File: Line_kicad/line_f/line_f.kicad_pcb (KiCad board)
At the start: 2 copper layers, 137.5 x 154 mm, 15 parts, among them M2 Motor_DC, M3 Motor_DC, SW1 SW_SPST, SW2 SW_SPDT, SW3 SW_Push, SW4 SW_Push, U1 TB6612FNG_LINE, m1 BLACKPILL

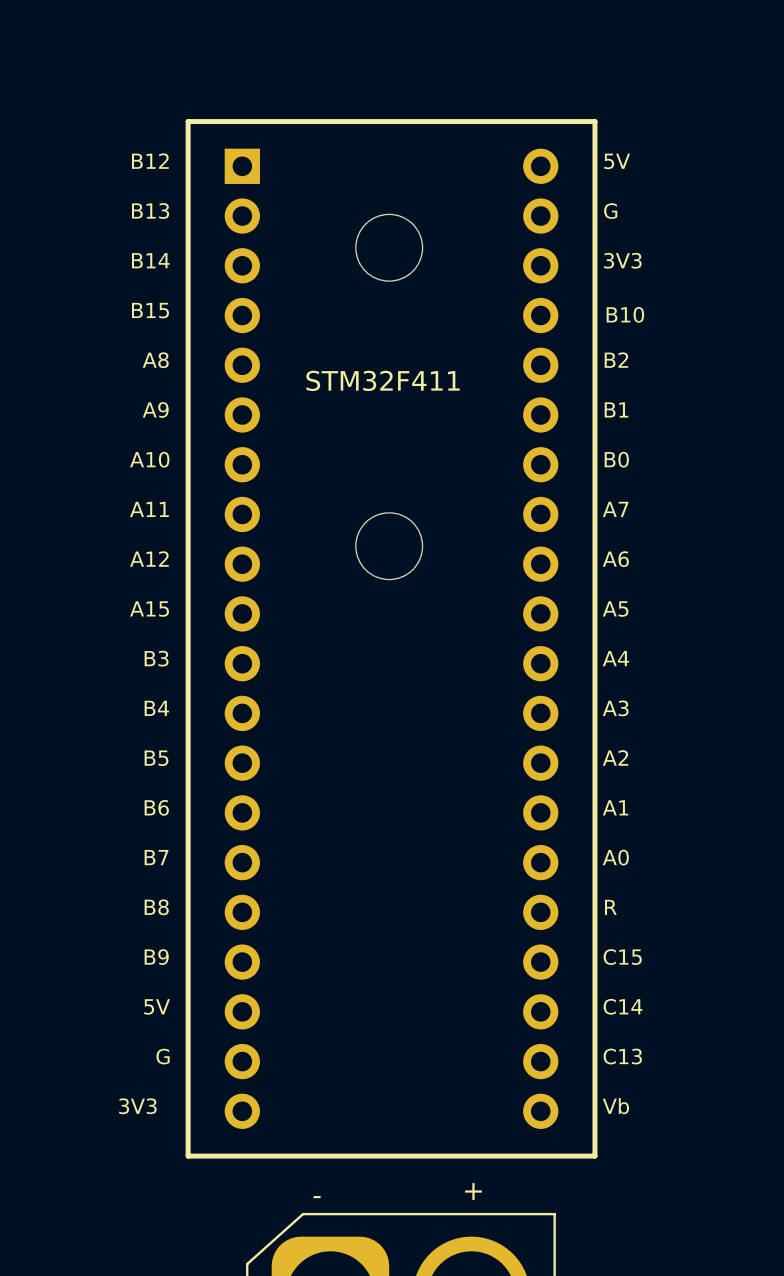
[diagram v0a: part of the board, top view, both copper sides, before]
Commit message: v9.0
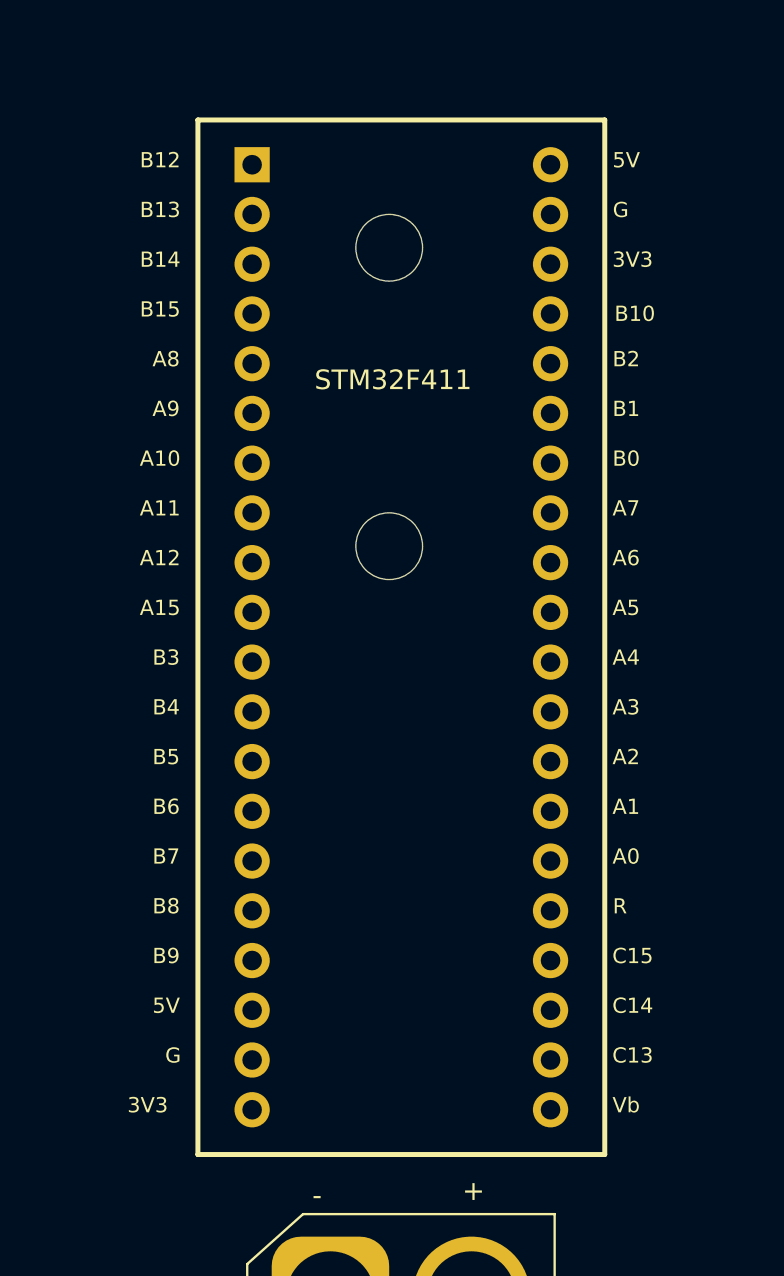
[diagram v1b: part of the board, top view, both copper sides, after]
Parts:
- moved m1 0.51 mm to (-75.9, 69.1)

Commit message: 6updatefrmsch#
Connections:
- LSA_UART1 pad 4: LSA_AN -> unconnected-(LSA_UART1-AN-Pad4)
- m1 pad 10: D3 -> LSA_UEN
- m1 pad 11: D4 -> PRIORITY_SW
- m1 pad 12: D5 -> JPULSE
- m1 pad 13: unconnected-(m1-B5-Pad13) -> SW_RUN
- m1 pad 16: D6 -> AI1
- m1 pad 17: D0 -> AI2
- m1 pad 19: unconnected-(m1-GND-Pad19) -> C_GND
- m1 pad 2: SW_RUN -> D3
- m1 pad 22: C_GND -> unconnected-(m1-GND-Pad22)
- m1 pad 26: D2 -> D6
- m1 pad 27: D1 -> D5
- m1 pad 28: LSA_AN -> D4
- m1 pad 29: BI2 -> PWMB
- m1 pad 3: LED_F -> D2
- m1 pad 30: BI1 -> BI2
- m1 pad 31: AI1 -> BI1
- m1 pad 32: AI2 -> LSA_TX
- m1 pad 33: PWMB -> LSA_RX
- m1 pad 4: SW_TRY -> D1
- m1 pad 5: JPULSE -> D0
- m1 pad 6: LSA_RX -> unconnected-(m1-A9-Pad6)
- m1 pad 7: LSA_TX -> unconnected-(m1-A10-Pad7)
- m1 pad 8: LSA_UEN -> SW_TRY
- m1 pad 9: PRIORITY_SW -> LED_F
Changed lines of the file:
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@@
 	(net 4 "5V")
 	(net 5 "Net-(D1-A)")
-	(net 6 "LSA_AN")
+	(net 6 "unconnected-(LSA_UART1-AN-Pad4)")
 	(net 7 "JPULSE")
 	(net 8 "D7")
@@
 	(net 15 "D2")
 	(net 16 "LSA_UEN")
-	(net 17 "unconnected-(m1-B5-Pad13)")
+	(net 17 "unconnected-(m1-A9-Pad6)")
 	(net 18 "unconnected-(LSA_UART1-Orphan-Pad8)")
 	(net 19 "unconnected-(LSA_UART1-Orphan1-Pad6)")
@@
 	(net 27 "unconnected-(m1-A0-Pad35)")
 	(net 28 "unconnected-(m1-C13-Pad39)")
-	(net 29 "unconnected-(m1-GND-Pad19)")
+	(net 29 "unconnected-(m1-GND-Pad22)")
 	(net 30 "BI1")
 	(net 31 "PWMA")
@@
 	(net 55 "unconnected-(U1-GND-Pad8)")
 	(net 56 "unconnected-(U1-GND-Pad3)")
+	(net 57 "unconnected-(m1-A10-Pad7)")
 	(footprint "LINE_F_FOOT_LIB:BATTERY_LINE_XT60"
 		(layer "F.Cu")
@@
 			)
 		)
-		(sheetname "Root")
+		(sheetname "/")
 		(sheetfile "line_f.kicad_sch")
 		(attr through_hole)
@@
 			)
 		)
-		(sheetname "Root")
+		(sheetname "/")
 		(sheetfile "line_f.kicad_sch")
 		(attr smd)
@@
 			)
 		)
-		(sheetname "Root")
+		(sheetname "/")
 		(sheetfile "line_f.kicad_sch")
 		(attr through_hole)
@@
 			)
 		)
+		(property "Sim.Pins" "1=K 2=A"
+			(at 0 0 0)
+			(unlocked yes)
+			(layer "F.Fab")
+			(hide yes)
+			(effects
+				(font
+					(size 1 1)
+					(thickness 0.15)
+				)
+			)
+		)
 		(property ki_fp_filters "LED* LED_SMD:* LED_THT:*")
-		(sheetname "Root")
+		(sheetname "/")
 		(sheetfile "line_f.kicad_sch")
 		(attr through_hole)
@@
 			)
 		)
-		(sheetname "Root")
+		(sheetname "/")
 		(sheetfile "line_f.kicad_sch")
 		(fp_line
@@
 			(layers "*.Cu" "*.Mask")
 			(remove_unused_layers no)
-			(net 44 "SW_RUN")
+			(net 13 "D3")
 			(pinfunction "B13")
 			(pintype "bidirectional")
@@
 			(layers "*.Cu" "*.Mask")
 			(remove_unused_layers no)
-			(net 42 "LED_F")
+			(net 15 "D2")
 			(pinfunction "B14")
 			(pintype "bidirectional")
@@
 			(layers "*.Cu" "*.Mask")
 			(remove_unused_layers no)
-			(net 41 "SW_TRY")
+			(net 12 "D1")
 			(pinfunction "B15")
 			(pintype "bidirectional")
@@
 			(layers "*.Cu" "*.Mask")
 			(remove_unused_layers no)
-			(net 7 "JPULSE")
+			(net 11 "D0")
 			(pinfunction "A8")
 			(pintype "bidirectional")
@@
 			(layers "*.Cu" "*.Mask")
 			(remove_unused_layers no)
-			(net 20 "LSA_RX")
+			(net 17 "unconnected-(m1-A9-Pad6)")
 			(pinfunction "A9")
-			(pintype "bidirectional")
+			(pintype "bidirectional+no_connect")
 			(solder_mask_margin 0.0508)
 			(thermal_bridge_angle 0)
@@
 			(layers "*.Cu" "*.Mask")
 			(remove_unused_layers no)
-			(net 22 "LSA_TX")
+			(net 57 "unconnected-(m1-A10-Pad7)")
 			(pinfunction "A10")
-			(pintype "bidirectional")
+			(pintype "bidirectional+no_connect")
 			(solder_mask_margin 0.0508)
 			(thermal_bridge_angle 0)
@@
 			(layers "*.Cu" "*.Mask")
 			(remove_unused_layers no)
-			(net 16 "LSA_UEN")
+			(net 41 "SW_TRY")
 			(pinfunction "A11")
 			(pintype "bidirectional")
@@
 			(layers "*.Cu" "*.Mask")
 			(remove_unused_layers no)
-			(net 23 "PRIORITY_SW")
+			(net 42 "LED_F")
 			(pinfunction "A12")
 			(pintype "bidirectional")
@@
 			(layers "*.Cu" "*.Mask")
 			(remove_unused_layers no)
-			(net 13 "D3")
+			(net 16 "LSA_UEN")
 			(pinfunction "A15")
 			(pintype "bidirectional")
@@
 			(layers "*.Cu" "*.Mask")
 			(remove_unused_layers no)
-			(net 10 "D4")
+			(net 23 "PRIORITY_SW")
 			(pinfunction "B3")
 			(pintype "bidirectional")
@@
 			(layers "*.Cu" "*.Mask")
 			(remove_unused_layers no)
-			(net 14 "D5")
+			(net 7 "JPULSE")
 			(pinfunction "B4")
 			(pintype "bidirectional")
@@
 			(layers "*.Cu" "*.Mask")
 			(remove_unused_layers no)
-			(net 17 "unconnected-(m1-B5-Pad13)")
+			(net 44 "SW_RUN")
 			(pinfunction "B5")
-			(pintype "no_connect")
+			(pintype "bidirectional")
 			(solder_mask_margin 0.0508)
 			(thermal_bridge_angle 0)
@@
 			(layers "*.Cu" "*.Mask")
 			(remove_unused_layers no)
-			(net 9 "D6")
+			(net 37 "AI1")
 			(pinfunction "B8")
 			(pintype "bidirectional")
@@
 			(layers "*.Cu" "*.Mask")
 			(remove_unused_layers no)
-			(net 11 "D0")
+			(net 38 "AI2")
 			(pinfunction "B9")
 			(pintype "bidirectional")
@@
 			(layers "*.Cu" "*.Mask")
 			(remove_unused_layers no)
-			(net 29 "unconnected-(m1-GND-Pad19)")
+			(net 1 "C_GND")
 			(pinfunction "GND")
-			(pintype "power_in+no_connect")
+			(pintype "power_in")
 			(solder_mask_margin 0.0508)
 			(thermal_bridge_angle 0)
@@
 			(layers "*.Cu" "*.Mask")
 			(remove_unused_layers no)
-			(net 1 "C_GND")
+			(net 29 "unconnected-(m1-GND-Pad22)")
 			(pinfunction "GND")
-			(pintype "power_in")
+			(pintype "power_in+no_connect")
 			(solder_mask_margin 0.0508)
 			(thermal_bridge_angle 0)
@@
 			(layers "*.Cu" "*.Mask")
 			(remove_unused_layers no)
-			(net 15 "D2")
+			(net 9 "D6")
 			(pinfunction "B1")
 			(pintype "bidirectional")
@@
 			(layers "*.Cu" "*.Mask")
 			(remove_unused_layers no)
-			(net 12 "D1")
+			(net 14 "D5")
 			(pinfunction "B0")
 			(pintype "bidirectional")
@@
 			(layers "*.Cu" "*.Mask")
 			(remove_unused_layers no)
-			(net 6 "LSA_AN")
+			(net 10 "D4")
 			(pinfunction "A7")
 			(pintype "bidirectional")
@@
 			(layers "*.Cu" "*.Mask")
 			(remove_unused_layers no)
-			(net 26 "BI2")
+			(net 33 "PWMB")
 			(pinfunction "A6")
 			(pintype "bidirectional")
@@
 			(layers "*.Cu" "*.Mask")
 			(remove_unused_layers no)
-			(net 30 "BI1")
+			(net 26 "BI2")
 			(pinfunction "A5")
 			(pintype "bidirectional")
@@
 			(layers "*.Cu" "*.Mask")
 			(remove_unused_layers no)
-			(net 37 "AI1")
+			(net 30 "BI1")
 			(pinfunction "A4")
 			(pintype "bidirectional")
@@
 			(layers "*.Cu" "*.Mask")
 			(remove_unused_layers no)
-			(net 38 "AI2")
+			(net 22 "LSA_TX")
 			(pinfunction "A3")
 			(pintype "bidirectional")
@@
 			(layers "*.Cu" "*.Mask")
 			(remove_unused_layers no)
-			(net 33 "PWMB")
+			(net 20 "LSA_RX")
 			(pinfunction "A2")
 			(pintype "bidirectional")
@@
 			(net 27 "unconnected-(m1-A0-Pad35)")
 			(pinfunction "A0")
-			(pintype "no_connect")
+			(pintype "bidirectional+no_connect")
 			(solder_mask_margin 0.0508)
 			(thermal_bridge_angle 0)
@@
 			)
 		)
-		(sheetname "Root")
+		(sheetname "/")
 		(sheetfile "line_f.kicad_sch")
 		(attr through_hole)
@@
 			(layers "*.Cu" "*.Mask")
 			(remove_unused_layers no)
-			(net 6 "LSA_AN")
+			(net 6 "unconnected-(LSA_UART1-AN-Pad4)")
 			(pinfunction "AN")
-			(pintype "bidirectional")
+			(pintype "bidirectional+no_connect")
 		)
 		(pad "5" thru_hole circle
@@
 		)
 		(property ki_fp_filters "PinHeader*P2.54mm* TerminalBlock*")
-		(sheetname "Root")
+		(sheetname "/")
 		(sheetfile "line_f.kicad_sch")
 		(attr through_hole)
@@
 			)
 		)
-		(sheetname "Root")
+		(sheetname "/")
 		(sheetfile "line_f.kicad_sch")
 		(attr through_hole)
@@
 			)
 		)
-		(sheetname "Root")
+		(sheetname "/")
 		(sheetfile "line_f.kicad_sch")
 		(fp_rect
@@
 			)
 		)
-		(sheetname "Root")
+		(sheetname "/")
 		(sheetfile "line_f.kicad_sch")
 		(attr through_hole)
@@
 			)
 		)
-		(sheetname "Root")
+		(sheetname "/")
 		(sheetfile "line_f.kicad_sch")
 		(attr through_hole)
@@
 			)
 		)
-		(sheetname "Root")
+		(sheetname "/")
 		(sheetfile "line_f.kicad_sch")
 		(attr through_hole)
@@
 			)
 		)
-		(sheetname "Root")
+		(sheetname "/")
 		(sheetfile "line_f.kicad_sch")
 		(attr through_hole)
@@
 		)
 		(property ki_fp_filters "R_*")
-		(sheetname "Root")
+		(sheetname "/")
 		(sheetfile "line_f.kicad_sch")
 		(attr through_hole)
@@
 		)
 		(property ki_fp_filters "PinHeader*P2.54mm* TerminalBlock*")
-		(sheetname "Root")
+		(sheetname "/")
 		(sheetfile "line_f.kicad_sch")
 		(attr through_hole)
